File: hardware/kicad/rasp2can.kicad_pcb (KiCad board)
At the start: 2 copper layers, 14 parts, among them P1 CONN_01X06, P2 CONN_01X03, U1 MCP2515, U2 MCP2551-I/P, Y1 16MHz

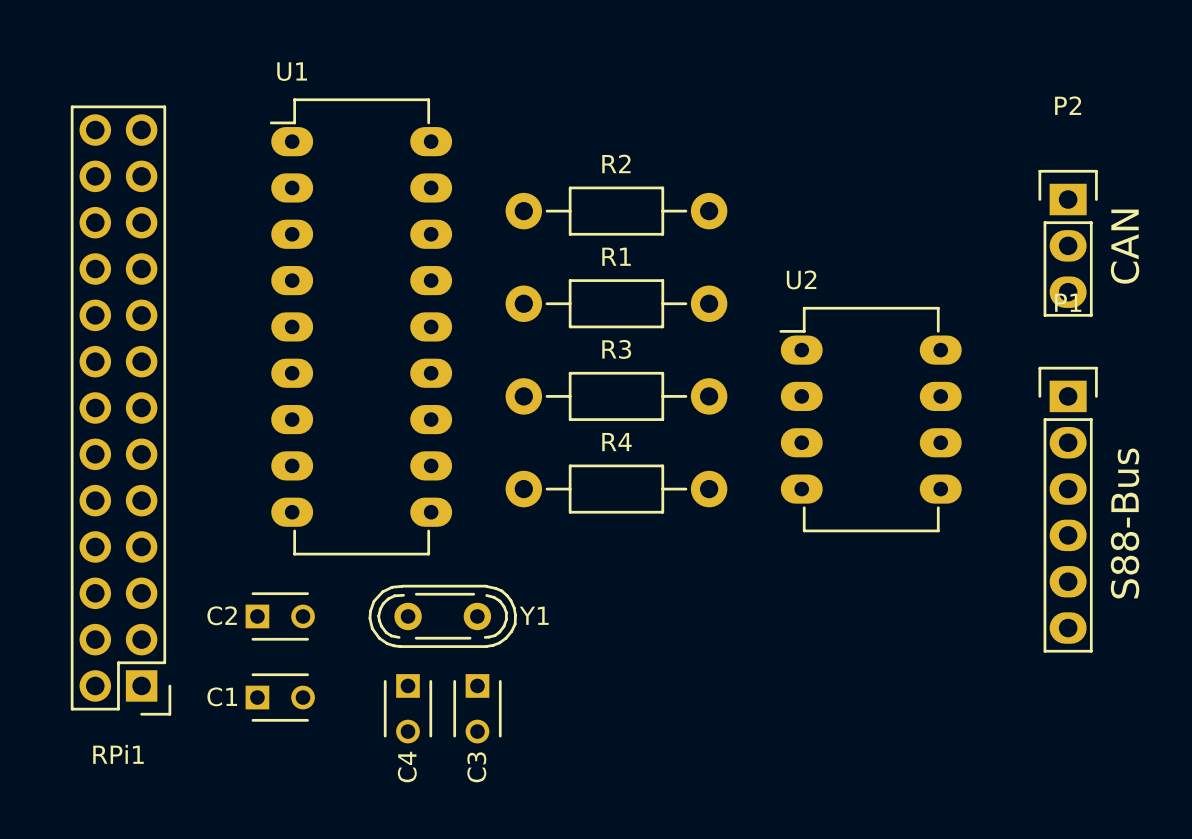
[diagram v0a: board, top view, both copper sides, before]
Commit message: update hardware
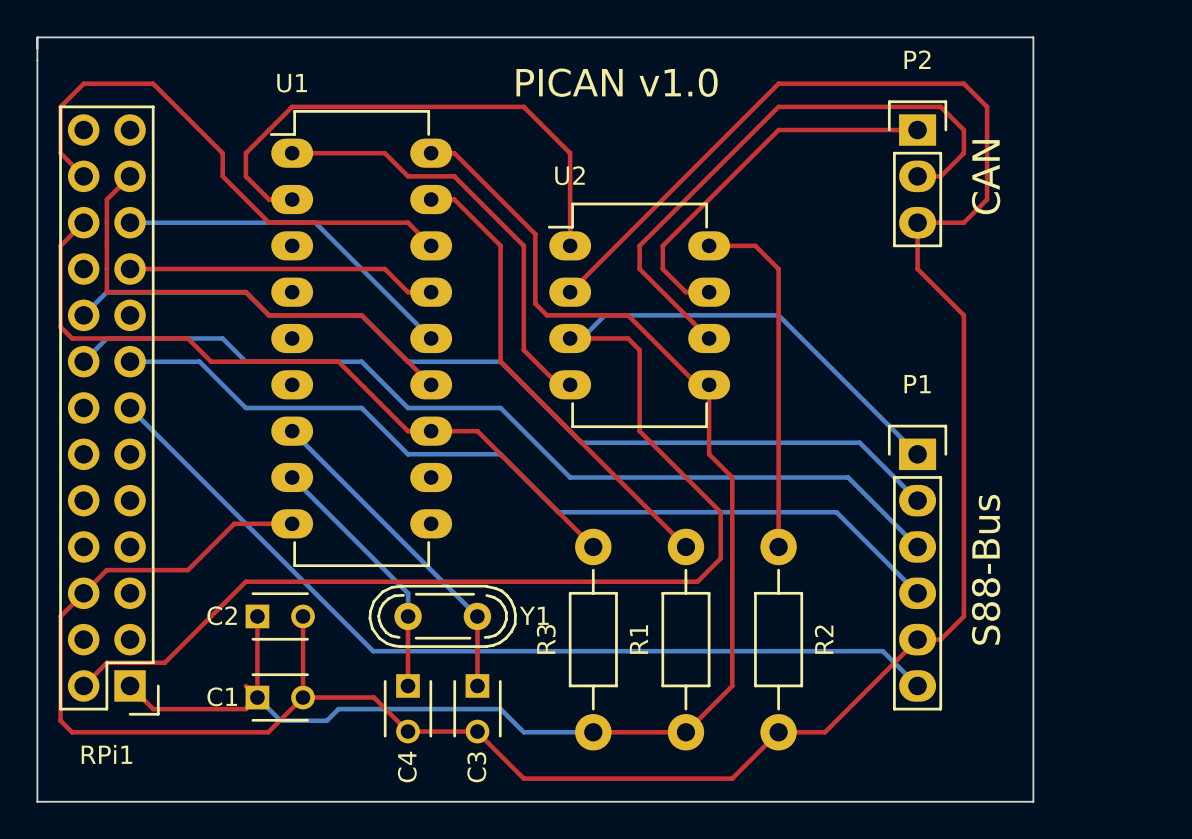
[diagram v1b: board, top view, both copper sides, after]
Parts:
- removed R4: 10k, Resistors_ThroughHole:Resistor_Horizontal_RM10mm
- U2: value MCP2551-I/P -> MCP2562
- moved R2 25.1 mm to (141.0, 92.7), turned to 270 degrees
- moved R1 18.8 mm to (135.9, 92.7), turned to 90 degrees
- moved U2 13.9 mm to (129.5, 71.1)
- moved R3 13.4 mm to (130.8, 92.7), turned to 270 degrees
- moved P2 9.09 mm to (148.6, 64.8)
- moved P1 8.84 mm to (148.6, 82.5)
- moved RPi1 0.64 mm to (105.4, 95.2)
- moved U1 0.64 mm to (114.3, 66.0)
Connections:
- R3 pad 1: GND -> Net-(R3-Pad1)
- R3 pad 2: Net-(R3-Pad2) -> +3V3
- RPi1 pad 22: Net-(RPi1-Pad22) -> Net-(R3-Pad1)
- U1 pad 12: Net-(RPi1-Pad22) -> Net-(R3-Pad1)
- U1 pad 2: Net-(R3-Pad2) -> Net-(U1-Pad2)
- U2 pad 1: Net-(U1-Pad1) -> Net-(U1-Pad2)
- U2 pad 4: Net-(R4-Pad2) -> Net-(U1-Pad1)
- U2 pad 5: (no net) -> +3V3
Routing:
- net GND: track 0.00 -> 141.9 mm
- net +3V3: track 0.00 -> 81.3 mm
- net +5V: track 0.00 -> 77.9 mm
- net /S88_RESET: track 0.00 -> 51.0 mm
- net /S88_PS: track 0.00 -> 51.0 mm
- net /S88_DATA: track 0.00 -> 49.5 mm
- net /S88_CLOCK: track 0.00 -> 48.4 mm
- net Net-(R3-Pad1): track 0.00 -> 40.4 mm
- net Net-(P2-Pad2): track 0.00 -> 32.5 mm
- net /SPI_CS: track 0.00 -> 29.6 mm
- net Net-(U1-Pad2): track 0.00 -> 29.3 mm
- net /SPI_CLK: track 0.00 -> 26.8 mm
- net Net-(R1-Pad2): track 0.00 -> 25.6 mm
- net Net-(U1-Pad1): track 0.00 -> 23.8 mm
- net Net-(P2-Pad1): track 0.00 -> 20.9 mm
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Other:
- board outline added: 54.6 x 41.9 mm
- board text added: "PICAN v1.0"
